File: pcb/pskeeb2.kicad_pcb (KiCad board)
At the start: 2 copper layers, 98 x 94.5 mm, 30 parts, among them J1 OLED, K11 KEYSW, K12 KEYSW, K13 KEYSW, K14 KEYSW, K15 KEYSW, K21 KEYSW, K22 KEYSW, K23 KEYSW, K24 KEYSW, K25 KEYSW, K31 KEYSW, K32 KEYSW, K33 KEYSW, K34 KEYSW, K35 KEYSW, K41 KEYSW, K42 KEYSW, K43 KEYSW, SW1 RotaryEncoder_Switch, SW2 RotaryEncoder_Switch, U1 wemos-esp32-s2-mini, U2 TRRS, U3 TRRS, U4 trackpoint

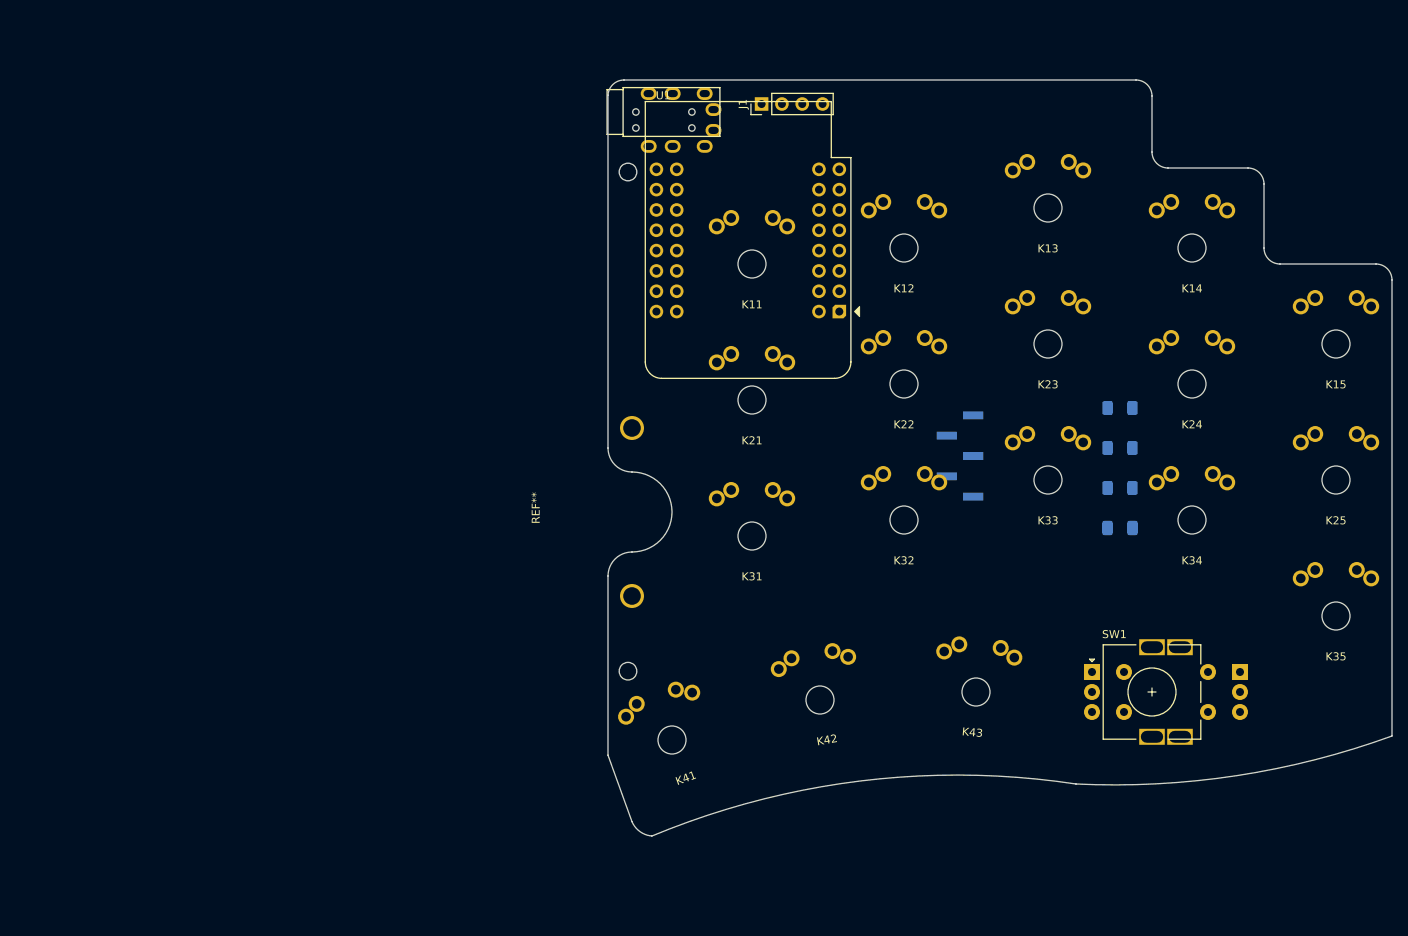
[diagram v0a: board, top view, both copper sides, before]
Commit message: feat: finish design
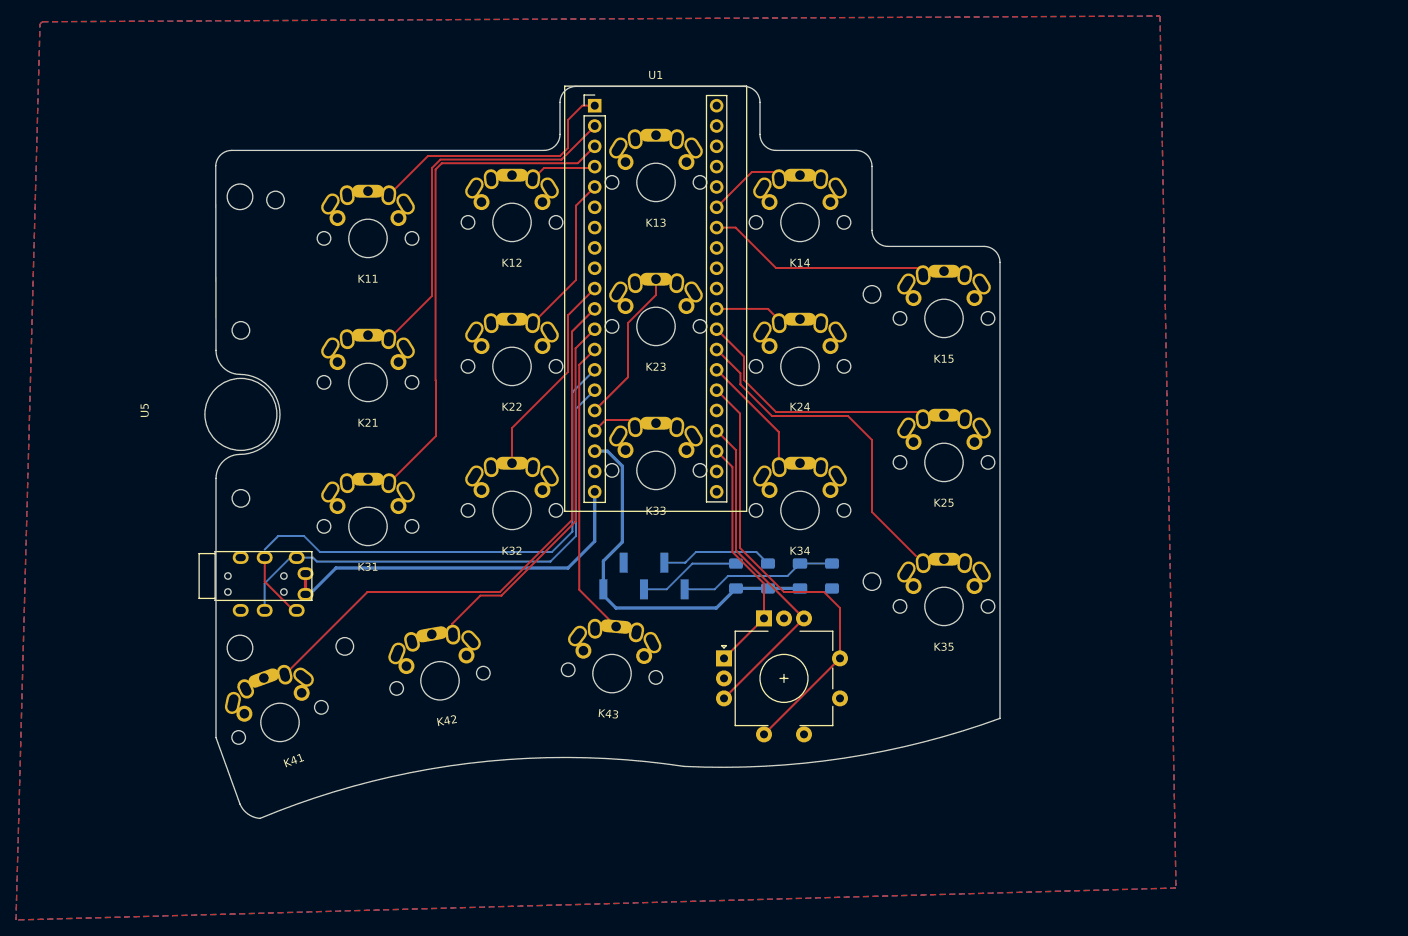
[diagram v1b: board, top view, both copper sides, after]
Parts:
- removed J1: OLED, Connector_PinHeader_2.54mm:PinHeader_1x04_P2.54mm_Vertical
- removed REF**: T400-Trackpoint, kwkb-footprint:T400-Trackpoint
- added U5: PlaceHoler, kwkb-footprint:T400-Trackpoint, F.Cu at (93.1, 89.8)
- K11, K12, K13, K14, K15, K21, K22, K23, K24, K25, K31, K32, K33, K34, K35, K41, K42, K43: footprint kwkb-footprint:Gateron Choc Reversible -> kwkb-footprint:Mx-Choc-Reversible
- SW1, SW2: footprint Rotary_Encoder:RotaryEncoder_Alps_EC11E-Switch_Vertical_H20mm -> Keebio-Parts:RotaryEncoder_EC11-no-legs
- U1: value wemos-esp32-s2-mini -> YAAJ_WeAct_BlackPill_Part_Like; footprint kwkb-footprint:WEMOS_S2_mini -> WeAct_BlackPill:YAAJ_WeAct_BlackPill_2
- moved U2 77.2 mm to (97.9, 110.0)
- moved U3 77.2 mm to (97.9, 112.0)
- moved SW2 57.0 mm to (169.0, 122.8), turned to -90 degrees
- moved R1 52.4 mm to (163.0, 110.0), turned to 90 degrees
- moved K12 49.1 mm to (135.0, 65.8)
- moved K13 49.1 mm to (153.0, 60.8)
- moved K14 49.1 mm to (171.0, 65.8)
- moved K15 49.1 mm to (189.0, 77.8)
- moved K22 49.0 mm to (135.0, 83.8)
- moved K23 49.0 mm to (153.0, 78.8)
- moved K24 49.0 mm to (171.0, 83.8)
- moved K25 49.0 mm to (189.0, 95.8)
- moved K41 49.0 mm to (106.0, 128.3)
- moved K32 49.0 mm to (135.0, 101.8)
- moved K33 49.0 mm to (153.0, 96.8)
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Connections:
- U1 pad 1: unconnected-(U1-Pad1) -> /k11
- U1 pad 10: unconnected-(U1-Pad10) -> /k32
- U1 pad 11: unconnected-(U1-Pad11) -> /k41
- U1 pad 12: unconnected-(U1-Pad12) -> /k42
- U1 pad 13: unconnected-(U1-Pad13) -> /k43
- U1 pad 14: unconnected-(U1-Pad14) -> TX
- U1 pad 15: unconnected-(U1-Pad15) -> RX
- U1 pad 16: +3V3 -> /k23
- U1 pad 17: +5V -> /k33
- U1 pad 18: unconnected-(U1-Pad18) -> +5V
- U1 pad 2: unconnected-(U1-Pad2) -> /k21
- U1 pad 20: GND -> +3V3
- U1 pad 23: unconnected-(U1-Pad23) -> ENA
- U1 pad 24: unconnected-(U1-Pad24) -> ENB
- U1 pad 26: unconnected-(U1-Pad26) -> /k44
- U1 pad 27: unconnected-(U1-Pad27) -> /k34
- U1 pad 28: unconnected-(U1-Pad28) -> /k35
- U1 pad 29: unconnected-(U1-Pad29) -> /k25
- U1 pad 3: unconnected-(U1-Pad3) -> /k31
- U1 pad 30: unconnected-(U1-Pad30) -> /k24
- U1 pad 4: unconnected-(U1-Pad4) -> /k12
- U1 pad 5: unconnected-(U1-Pad5) -> /k22
- U2 pad 1: (no net) -> +3V3
- U2 pad 2: (no net) -> RX
- U2 pad 3: (no net) -> TX
- U2 pad 4: (no net) -> GND
- U3 pad 1: (no net) -> +3V3
- U3 pad 2: (no net) -> TX
- U3 pad 3: (no net) -> RX
- U3 pad 4: (no net) -> GND
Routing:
- net /k41: track 0.00 -> 71.5 mm
- net TX: track 0.00 -> 70.9 mm
- net RX: track 0.00 -> 64.4 mm
- net /k31: track 0.00 -> 62.8 mm
- net /k44: track 0.00 -> 56.3 mm
- net +3V3: track 0.00 -> 47.7 mm
- net +5V: track 0.00 -> 47.6 mm
- net /k42: track 0.00 -> 47.2 mm
- net /k21: track 0.00 -> 46.2 mm
- net ENB: track 0.00 -> 42.1 mm
- net /k35: track 0.00 -> 41.7 mm
- net /k43: track 0.00 -> 37.4 mm
- net /k11: track 0.00 -> 35.2 mm
- net /k25: track 0.00 -> 32.0 mm
- net ENA: track 0.00 -> 30.4 mm
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- added copper zone on B.Cu, net GND
- added copper zone on F.Cu, net GND
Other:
- board size 98 x 94.5 mm -> 98 x 91.5 mm
- board text added: "100k/2.2uF/4.7k/4.7k"
- board text added: "R/D/C/G/V"
